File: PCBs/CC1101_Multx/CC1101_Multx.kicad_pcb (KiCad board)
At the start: 4 copper layers, 41 x 26.6 mm, 45 parts, among them IC1 CC1101RGPR, IC2 ASWD-S2-0005-T, IC3 ASWD-S2-0005-T, IC4 ASWD-S2-0005-T, J1 MCU, J2 MCU, J3 MCU, J4 MCU, J5 MCU, J6 MCU, J7 MCU, J8 MCU, J9 MCU, Y1 XRCGB26M000F1S2BR0

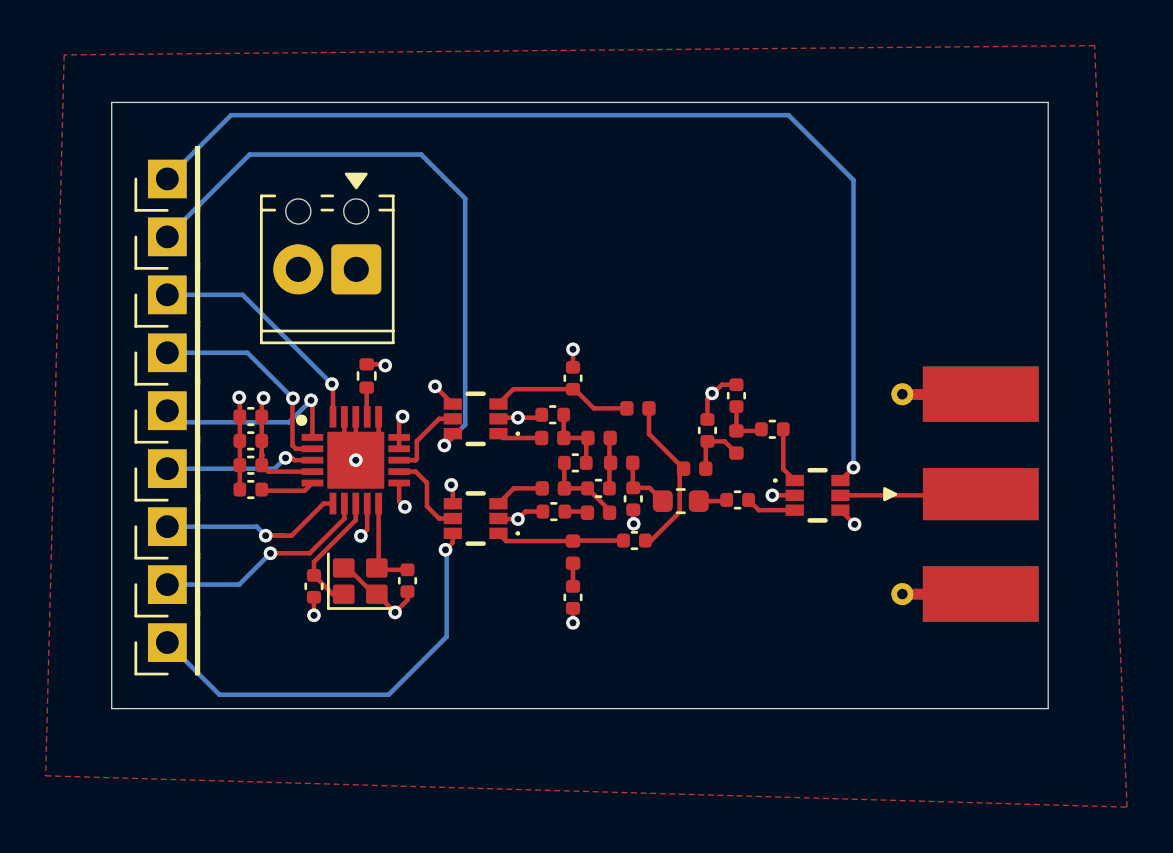
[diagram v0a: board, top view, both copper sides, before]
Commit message: layout2
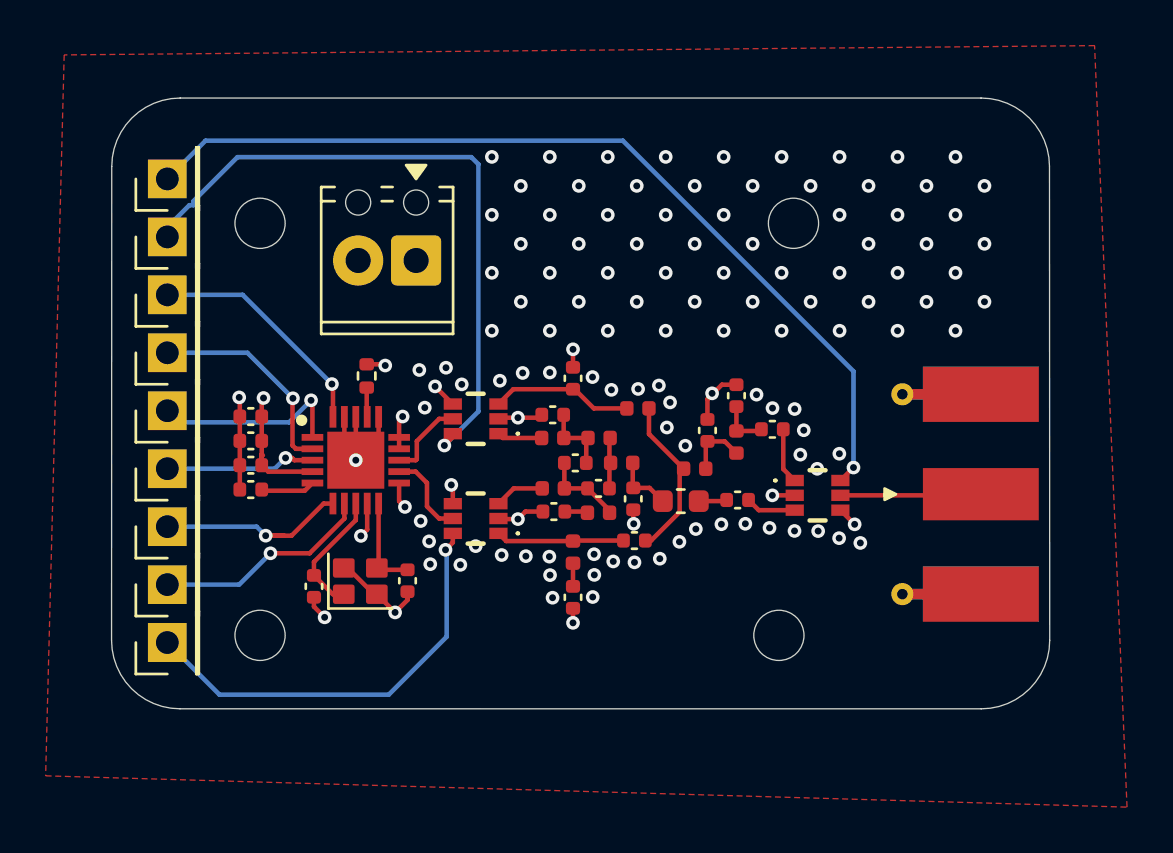
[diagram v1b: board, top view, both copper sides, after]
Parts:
- added REF**: MountingHole_2.2mm_M2_DIN965, MountingHole:MountingHole_2.2mm_M2_DIN965, F.Cu at (152.4, 89.5)
- added REF**: MountingHole_2.2mm_M2_DIN965, MountingHole:MountingHole_2.2mm_M2_DIN965, F.Cu at (152.4, 71.5)
- added REF**: MountingHole_2.2mm_M2_DIN965, MountingHole:MountingHole_2.2mm_M2_DIN965, F.Cu at (175.1, 89.5)
- added REF**: MountingHole_2.2mm_M2_DIN965, MountingHole:MountingHole_2.2mm_M2_DIN965, F.Cu at (175.8, 71.5)
- moved BT1 2.65 mm to (159.2, 73.1)
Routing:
- net Net-(IC4-VCTL): track 45.8 -> 40.0 mm
- net Net-(IC2-VCTL): track 27.2 -> 29.2 mm
- net /AGND: track 25.7 -> 26.0 mm, vias 12 -> 119
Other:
- board size 41 x 26.6 mm -> 41.1 x 26.8 mm

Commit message: Layout V
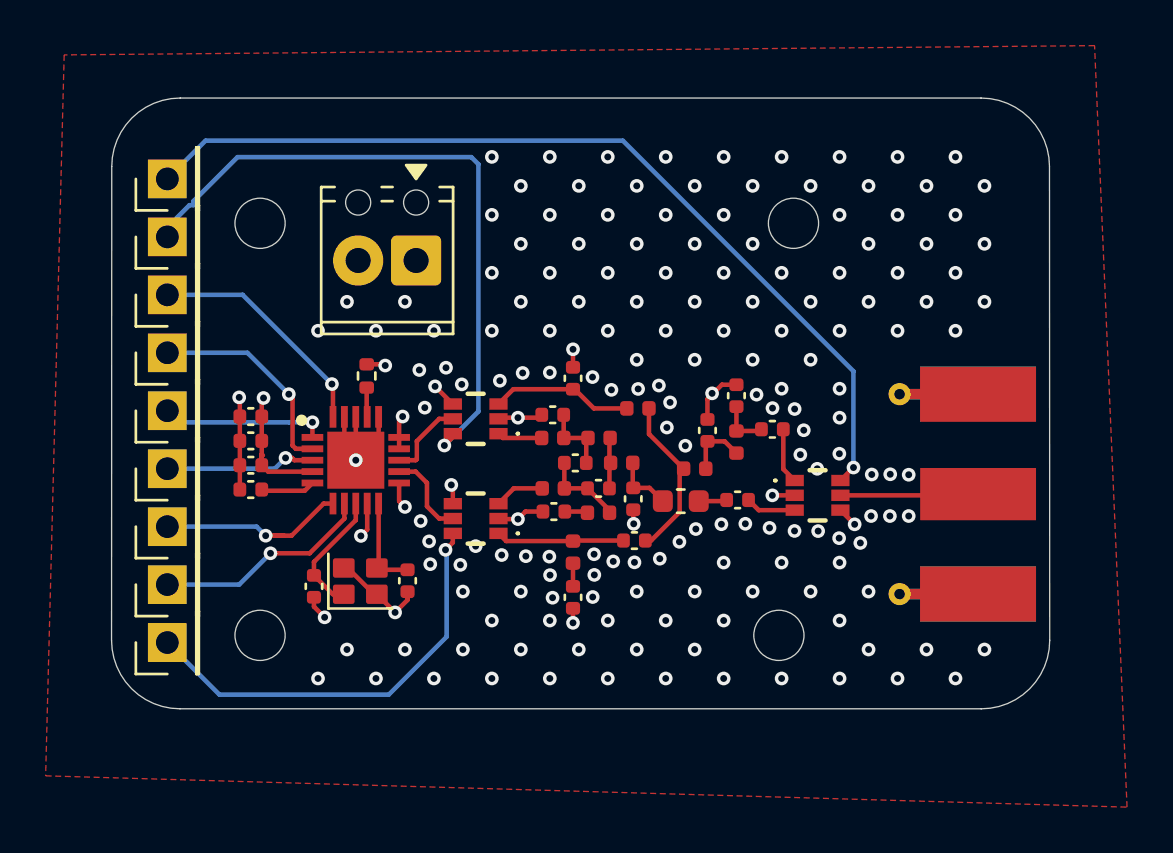
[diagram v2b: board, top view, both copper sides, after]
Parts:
- moved AE1 0.12 mm to (182.2, 83.4)
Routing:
- net Net-(IC1-SCLK): track 8.63 -> 7.24 mm
- net /AGND: vias 119 -> 175
